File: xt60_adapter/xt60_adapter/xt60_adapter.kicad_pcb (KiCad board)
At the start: 2 copper layers, 30.5 x 65.9 mm, 3 parts, among them J1 Barrel_Jack_Switch, J2 Conn_01x02

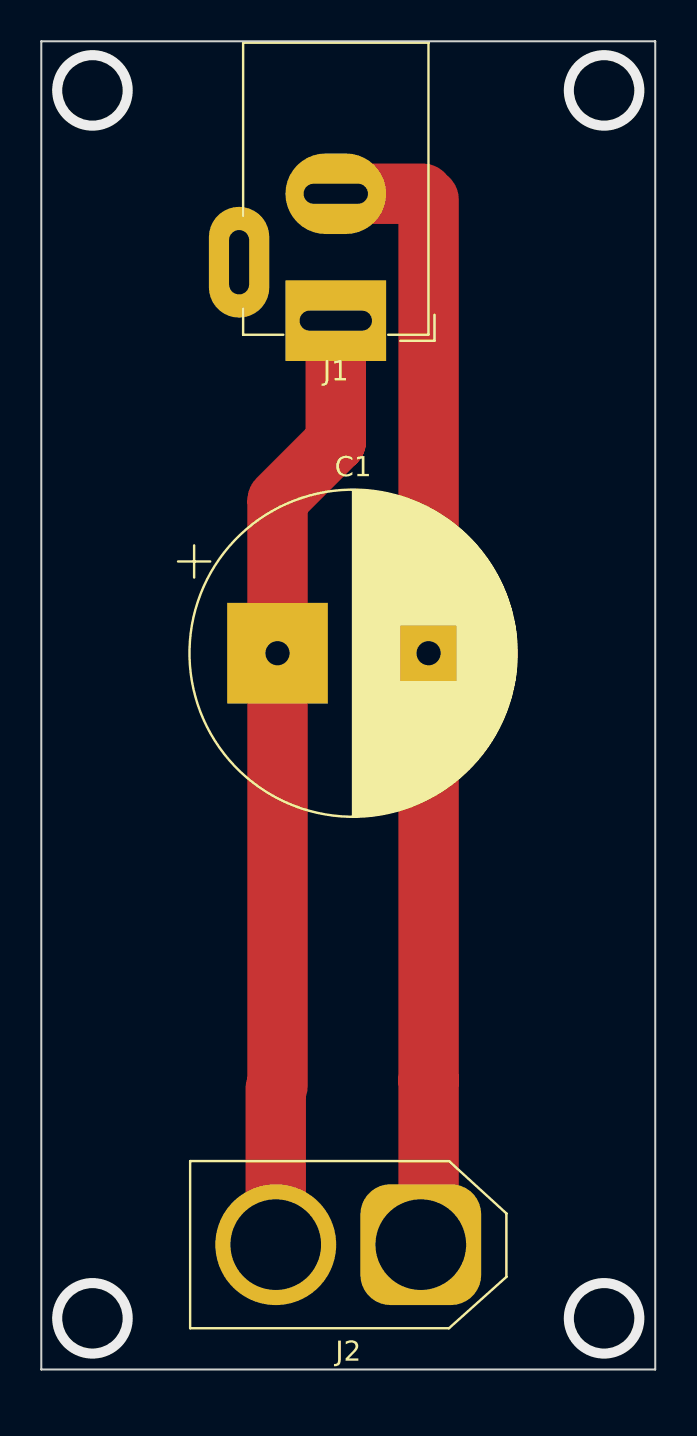
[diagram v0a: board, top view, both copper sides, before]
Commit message: Add projects
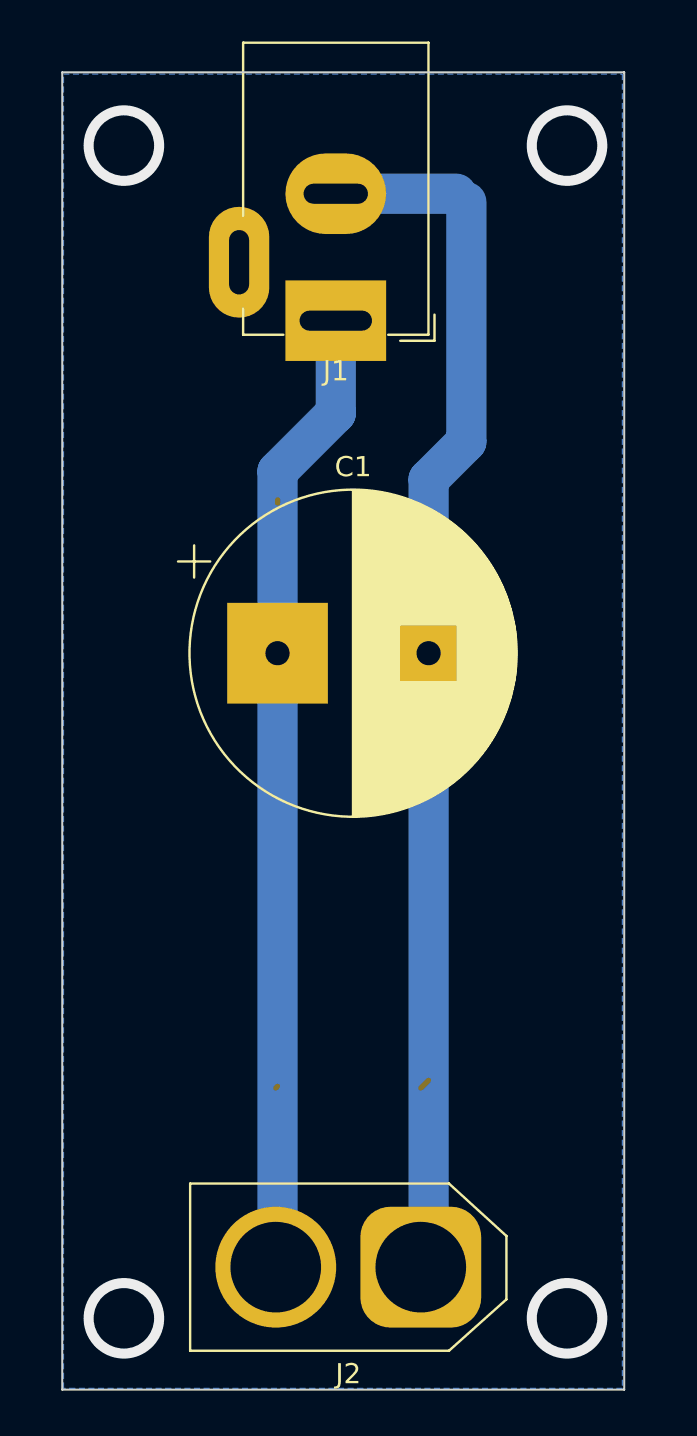
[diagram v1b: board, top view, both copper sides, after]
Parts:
- moved J2 1.12 mm to (107.7, 106.7)
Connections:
- net Net-(C1-Pad2) renamed GND
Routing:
- net GND: track 57.3 -> 61.0 mm
- net Net-(C1-Pad1): track 47.1 -> 48.5 mm
- net (no net): track 0.00 -> 0.55 mm
- added copper zone on B.Cu, net GND
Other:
- board size 30.5 x 65.9 mm -> 27.9 x 65.4 mm
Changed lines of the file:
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@@
   (net 0 "")
   (net 1 "Net-(C1-Pad1)")
-  (net 2 "Net-(C1-Pad2)")
+  (net 2 "GND")
   (net 3 "unconnected-(J1-Pad3)")
   (footprint "Connector_BarrelJack:BarrelJack_GCT_DCJ200-10-A_Horizontal" (layer "F.Cu")
@@
     (descr "Barrel jack connector (5.5 mm outer diameter, 2.05 inner diameter ), https://gct.co/files/drawings/dcj200-10.pdf")
     (tags "connector barrel jack")
-    (property "Sheetfile" "File: xt60_adapter.kicad_sch")
+    (property "Sheetfile" "xt60_adapter.kicad_sch")
     (property "Sheetname" "")
     (attr through_hole)
@@
       (net 1 "Net-(C1-Pad1)") (pintype "passive"))
     (pad "2" thru_hole oval (at 0 6.3 180) (size 5 4) (drill oval 3.2 1) (layers *.Cu *.Mask)
-      (net 2 "Net-(C1-Pad2)") (pintype "passive"))
+      (net 2 "GND") (pintype "passive"))
     (pad "3" thru_hole oval (at 4.8 2.9 180) (size 3 5.5) (drill oval 1 3.2) (layers *.Cu *.Mask)
       (net 3 "unconnected-(J1-Pad3)") (pintype "passive"))
@@
     (descr "CP, Radial series, Radial, pin pitch=7.50mm, , diameter=16mm, Electrolytic Capacitor")
     (tags "CP Radial series Radial pin pitch 7.50mm  diameter 16mm Electrolytic Capacitor")
-    (property "Sheetfile" "File: xt60_adapter.kicad_sch")
+    (property "Sheetfile" "xt60_adapter.kicad_sch")
     (property "Sheetname" "")
     (attr through_hole)
@@
       (net 1 "Net-(C1-Pad1)") (pintype "passive"))
     (pad "2" thru_hole circle (at 7.5 0) (size 5 5) (drill 1.2) (layers *.Cu *.Mask)
-      (net 2 "Net-(C1-Pad2)") (pintype "passive"))
+      (net 2 "GND") (pintype "passive"))
     (model "${KICAD6_3DMODEL_DIR}/Capacitor_THT.3dshapes/CP_Radial_D16.0mm_P7.50mm.wrl"
       (offset (xyz 0 0 0))
@@
   )
   (footprint "Connector_AMASS:AMASS_XT60-M_1x02_P7.20mm_Vertical" (layer "F.Cu")
-    (at 107.74 105.5624 180)
+    (at 107.74 106.68 180)
     (descr "AMASS female XT60, through hole, vertical, https://www.tme.eu/Document/2d152ced3b7a446066e6c419d84bb460/XT60%20SPEC.pdf")
     (tags "XT60 female vertical")
-    (property "Sheetfile" "File: xt60_adapter.kicad_sch")
+    (property "Sheetfile" "xt60_adapter.kicad_sch")
     (property "Sheetname" "")
     (attr through_hole)
@@
     (fp_line (start -1.4 4.05) (end 11.35 4.05) (layer "F.Fab") (width 0.12))
     (pad "1" thru_hole roundrect (at 0 0 180) (size 6 6) (drill 4.5) (layers *.Cu *.Mask) (roundrect_rratio 0.25)
-      (net 2 "Net-(C1-Pad2)") (pinfunction "Pin_1") (pintype "passive"))
+      (net 2 "GND") (pinfunction "Pin_1") (pintype "passive"))
     (pad "2" thru_hole circle (at 7.2 0 180) (size 6 6) (drill 4.5) (layers *.Cu *.Mask)
       (net 1 "Net-(C1-Pad1)") (pinfunction "Pin_2") (pintype "passive"))
@@
     )
   )
-  (gr_rect (start 88.9 45.8216) (end 119.38 111.76) (layer "Edge.Cuts") (width 0.1) (fill none))
-  (via (at 116.84 48.26) (size 4) (drill 3) (layers "F.Cu" "B.Cu") (free) (net 0))
-  (via (at 91.44 48.26) (size 4) (drill 3) (layers "F.Cu" "B.Cu") (free) (net 0))
-  (via (at 91.44 109.22) (size 4) (drill 3) (layers "F.Cu" "B.Cu") (free) (net 0))
-  (via (at 116.84 109.22) (size 4) (drill 3) (layers "F.Cu" "B.Cu") (free) (net 0))
-  (segment (start 100.627246 76.2) (end 100.627246 97.702754) (width 3) (layer "F.Cu") (net 1))
-  (segment (start 100.627246 68.739954) (end 100.627246 76.2) (width 3) (layer "F.Cu") (net 1))
-  (segment (start 100.54 97.79) (end 100.54 105.5624) (width 3) (layer "F.Cu") (net 1))
+  (gr_rect (start 89.94 47.3616) (end 117.84 112.76) (layer "Edge.Cuts") (width 0.1) (fill none))
+  (segment (start 107.74 97.79) (end 108.127246 97.402754) (width 0.25) (layer "F.Cu") (net 0))
+  (via (at 115 51) (size 4) (drill 3) (layers "F.Cu" "B.Cu") (free) (net 0))
+  (via (at 93 51) (size 4) (drill 3) (layers "F.Cu" "B.Cu") (free) (net 0))
+  (via (at 93 109.22) (size 4) (drill 3) (layers "F.Cu" "B.Cu") (free) (net 0))
+  (via (at 115 109.22) (size 4) (drill 3) (layers "F.Cu" "B.Cu") (free) (net 0))
   (segment (start 100.6348 68.7324) (end 100.627246 68.739954) (width 0.25) (layer "F.Cu") (net 1))
-  (segment (start 103.52 65.6948) (end 100.6348 68.58) (width 3) (layer "F.Cu") (net 1))
-  (segment (start 103.52 59.69) (end 103.52 65.6948) (width 3) (layer "F.Cu") (net 1))
   (segment (start 100.6348 68.58) (end 100.6348 68.7324) (width 0.25) (layer "F.Cu") (net 1))
   (segment (start 100.627246 97.702754) (end 100.54 97.79) (width 0.25) (layer "F.Cu") (net 1))
-  (segment (start 107.8476 53.39) (end 108.127246 53.669646) (width 0.25) (layer "F.Cu") (net 2))
-  (segment (start 108.127246 97.402754) (end 108.127246 105.175154) (width 3) (layer "F.Cu") (net 2))
-  (segment (start 108.127246 53.669646) (end 108.127246 76.2) (width 3) (layer "F.Cu") (net 2))
-  (segment (start 108.127246 97.402754) (end 108.127246 76.2) (width 3) (layer "F.Cu") (net 2))
-  (segment (start 107.74 97.79) (end 108.127246 97.402754) (width 0.25) (layer "F.Cu") (net 2))
-  (segment (start 103.52 53.39) (end 107.8476 53.39) (width 3) (layer "F.Cu") (net 2))
+  (segment (start 100.627246 76.2) (end 100.627246 106.592754) (width 2) (layer "B.Cu") (net 1))
+  (segment (start 103.52 64.28) (end 100.627246 67.172754) (width 2) (layer "B.Cu") (net 1))
+  (segment (start 100.627246 67.172754) (end 100.627246 76.2) (width 2) (layer "B.Cu") (net 1))
+  (segment (start 103.52 59.69) (end 103.52 64.28) (width 2) (layer "B.Cu") (net 1))
+  (segment (start 100.627246 106.592754) (end 100.54 106.68) (width 0.25) (layer "B.Cu") (net 1))
   (segment (start 108.127246 105.175154) (end 107.74 105.5624) (width 0.25) (layer "F.Cu") (net 2))
+  (segment (start 110 65.7) (end 110 53.8) (width 2) (layer "B.Cu") (net 2))
+  (segment (start 108.127246 67.572754) (end 110 65.7) (width 2) (layer "B.Cu") (net 2))
+  (segment (start 109.55 53.35) (end 109.51 53.39) (width 0.25) (layer "B.Cu") (net 2))
+  (segment (start 110 53.8) (end 109.55 53.35) (width 0.25) (layer "B.Cu") (net 2))
+  (segment (start 109.51 53.39) (end 103.52 53.39) (width 2) (layer "B.Cu") (net 2))
+  (segment (start 108.127246 76.2) (end 108.127246 67.572754) (width 2) (layer "B.Cu") (net 2))
+  (segment (start 108.127246 76.2) (end 108.127246 106.292754) (width 2) (layer "B.Cu") (net 2))
+  (segment (start 108.127246 106.292754) (end 107.74 106.68) (width 0.25) (layer "B.Cu") (net 2))
+  (zone (net 2) (net_name "GND") (layer "B.Cu") (hatch edge 0.508)
+    (connect_pads (clearance 0.508))
+    (min_thickness 0.254) (filled_areas_thickness no)
+    (fill yes (thermal_gap 0.508) (thermal_bridge_width 0.508))
+    (polygon
+      (pts
+        (xy 117.75 112.7)
+        (xy 90 112.7)
+        (xy 90 47.45)
+        (xy 117.75 47.45)
+      )
+    )
+  )
 )
